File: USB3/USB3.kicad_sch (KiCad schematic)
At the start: 1 part, among them U8 TUSB8020BIPHPRQ1

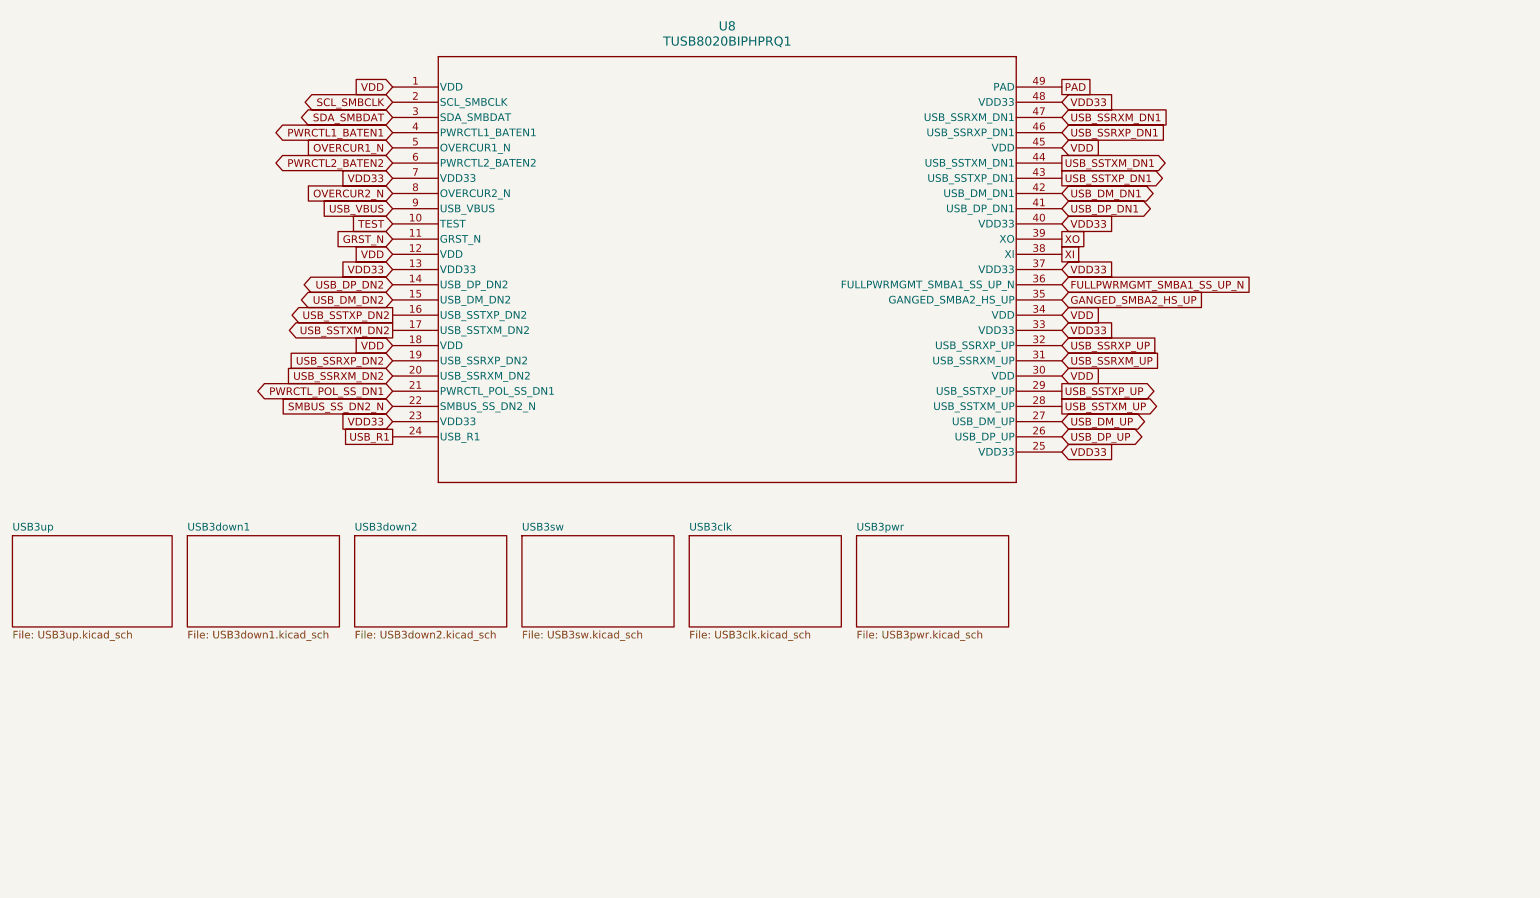
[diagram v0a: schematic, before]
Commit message: usb3 work cont
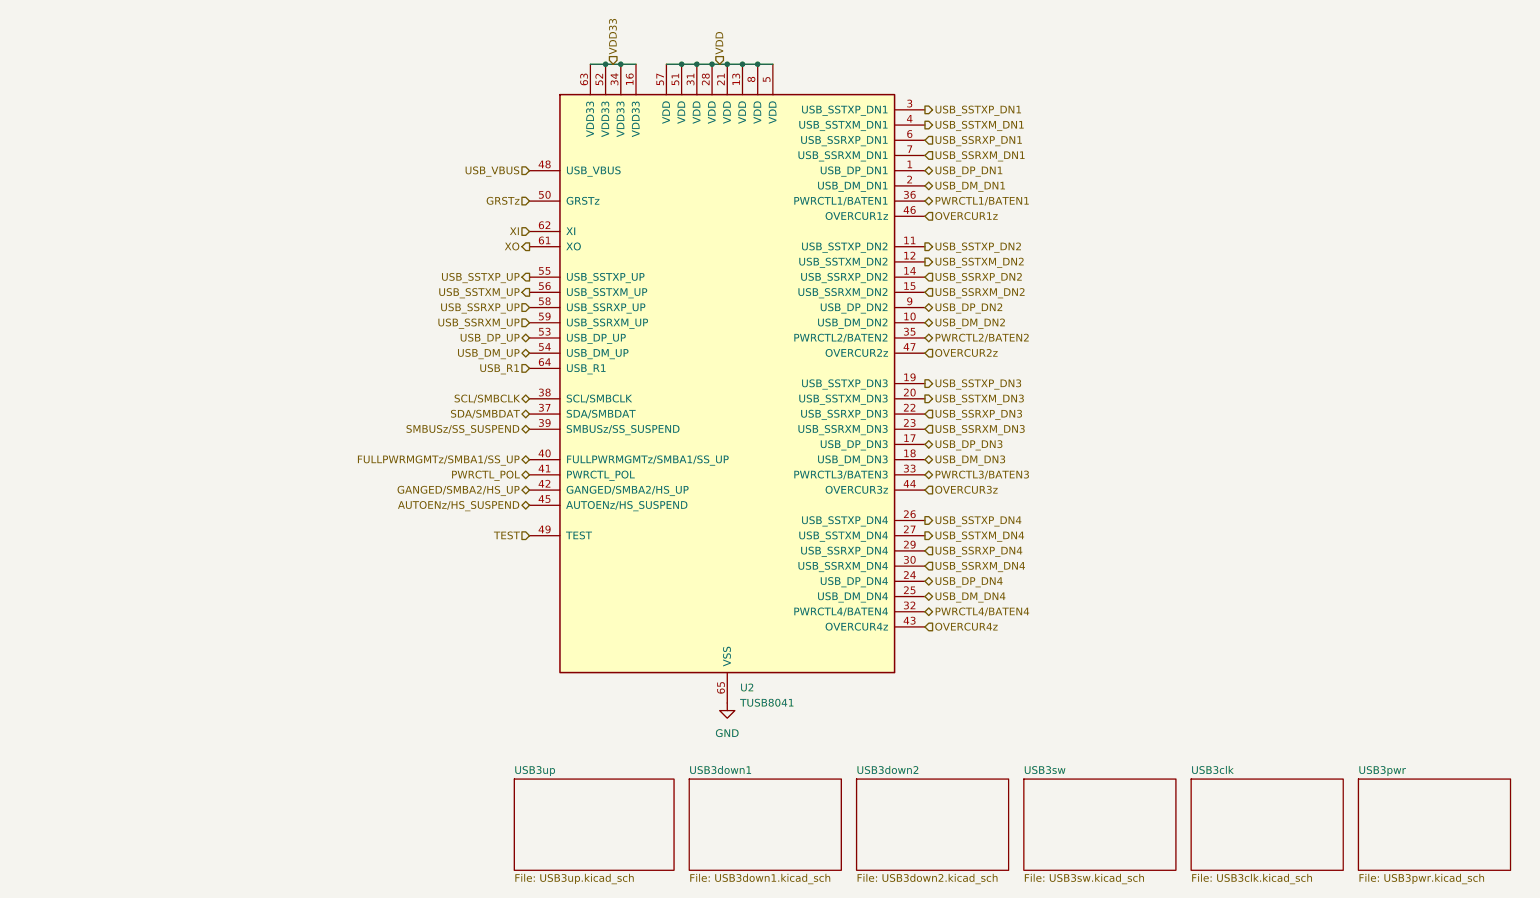
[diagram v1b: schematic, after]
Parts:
- removed U8: TUSB8020BIPHPRQ1, PHP0048E_N_TEX, symbol 2025-10-11_06-29-10:TUSB8020BIPHPRQ1
- added U2: TUSB8041, Package_DFN_QFN:QFN-64-1EP_9x9mm_P0.5mm_EP6x6mm_ThermalVias, symbol Interface_USB:TUSB8041
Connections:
- net TEST: now also U2.49 (TEST)
- net USB_DM_DN1: now also U2.2 (USB_DM_DN1)
- net USB_DM_DN2: now also U2.10 (USB_DM_DN2)
- net USB_DM_UP: now also U2.54 (USB_DM_UP)
- net USB_DP_DN1: now also U2.1 (USB_DP_DN1)
- net USB_DP_DN2: now also U2.9 (USB_DP_DN2)
- net USB_DP_UP: now also U2.53 (USB_DP_UP)
- net USB_R1: now also U2.64 (USB_R1)
- net USB_SSRXM_DN1: now also U2.7 (USB_SSRXM_DN1)
- net USB_SSRXM_DN2: now also U2.15 (USB_SSRXM_DN2)
- net USB_SSRXM_UP: now also U2.59 (USB_SSRXM_UP)
- net USB_SSRXP_DN1: now also U2.6 (USB_SSRXP_DN1)
- net USB_SSRXP_DN2: now also U2.14 (USB_SSRXP_DN2)
- net USB_SSRXP_UP: now also U2.58 (USB_SSRXP_UP)
- net USB_SSTXM_DN1: now also U2.4 (USB_SSTXM_DN1)
- net USB_SSTXM_DN2: now also U2.12 (USB_SSTXM_DN2)
- net USB_SSTXM_UP: now also U2.56 (USB_SSTXM_UP)
- net USB_SSTXP_DN1: now also U2.3 (USB_SSTXP_DN1)
- net USB_SSTXP_DN2: now also U2.11 (USB_SSTXP_DN2)
- net USB_SSTXP_UP: now also U2.55 (USB_SSTXP_UP)
- net USB_VBUS: now also U2.48 (USB_VBUS)
- net VDD: now also U2.13 (VDD), U2.21 (VDD), U2.28 (VDD), U2.31 (VDD), U2.5 (VDD), U2.51 (VDD), U2.57 (VDD), U2.8 (VDD)
- net VDD33: now also U2.16 (VDD33), U2.34 (VDD33), U2.52 (VDD33), U2.63 (VDD33)
- net XI: now also U2.62 (XI)
- net XO: now also U2.61 (XO)
- new net AUTOENz/HS_SUSPEND: U2.45 (AUTOENz/HS_SUSPEND)
- new net FULLPWRMGMTz/SMBA1/SS_UP: U2.40 (FULLPWRMGMTz/SMBA1/SS_UP)
- new net GANGED/SMBA2/HS_UP: U2.42 (GANGED/SMBA2/HS_UP)
- new net GND: U2.65 (VSS)
- new net GRSTz: U2.50 (GRSTz)
- new net OVERCUR1z: U2.46 (OVERCUR1z)
- new net OVERCUR2z: U2.47 (OVERCUR2z)
- new net OVERCUR3z: U2.44 (OVERCUR3z)
- new net OVERCUR4z: U2.43 (OVERCUR4z)
- new net PWRCTL1/BATEN1: U2.36 (PWRCTL1/BATEN1)
- new net PWRCTL2/BATEN2: U2.35 (PWRCTL2/BATEN2)
- new net PWRCTL3/BATEN3: U2.33 (PWRCTL3/BATEN3)
- new net PWRCTL4/BATEN4: U2.32 (PWRCTL4/BATEN4)
- new net PWRCTL_POL: U2.41 (PWRCTL_POL)
- new net SCL/SMBCLK: U2.38 (SCL/SMBCLK)
- new net SDA/SMBDAT: U2.37 (SDA/SMBDAT)
- new net SMBUSz/SS_SUSPEND: U2.39 (SMBUSz/SS_SUSPEND)
- new net USB_DM_DN3: U2.18 (USB_DM_DN3)
- new net USB_DM_DN4: U2.25 (USB_DM_DN4)
- new net USB_DP_DN3: U2.17 (USB_DP_DN3)
- new net USB_DP_DN4: U2.24 (USB_DP_DN4)
- new net USB_SSRXM_DN3: U2.23 (USB_SSRXM_DN3)
- new net USB_SSRXM_DN4: U2.30 (USB_SSRXM_DN4)
- new net USB_SSRXP_DN3: U2.22 (USB_SSRXP_DN3)
- new net USB_SSRXP_DN4: U2.29 (USB_SSRXP_DN4)
- new net USB_SSTXM_DN3: U2.20 (USB_SSTXM_DN3)
- new net USB_SSTXM_DN4: U2.27 (USB_SSTXM_DN4)
- new net USB_SSTXP_DN3: U2.19 (USB_SSTXP_DN3)
- new net USB_SSTXP_DN4: U2.26 (USB_SSTXP_DN4)
